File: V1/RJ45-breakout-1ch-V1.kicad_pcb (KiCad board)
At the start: 2 copper layers, 110 x 100 mm, 37 parts, among them J1 RJ45, J2 SWITCHES

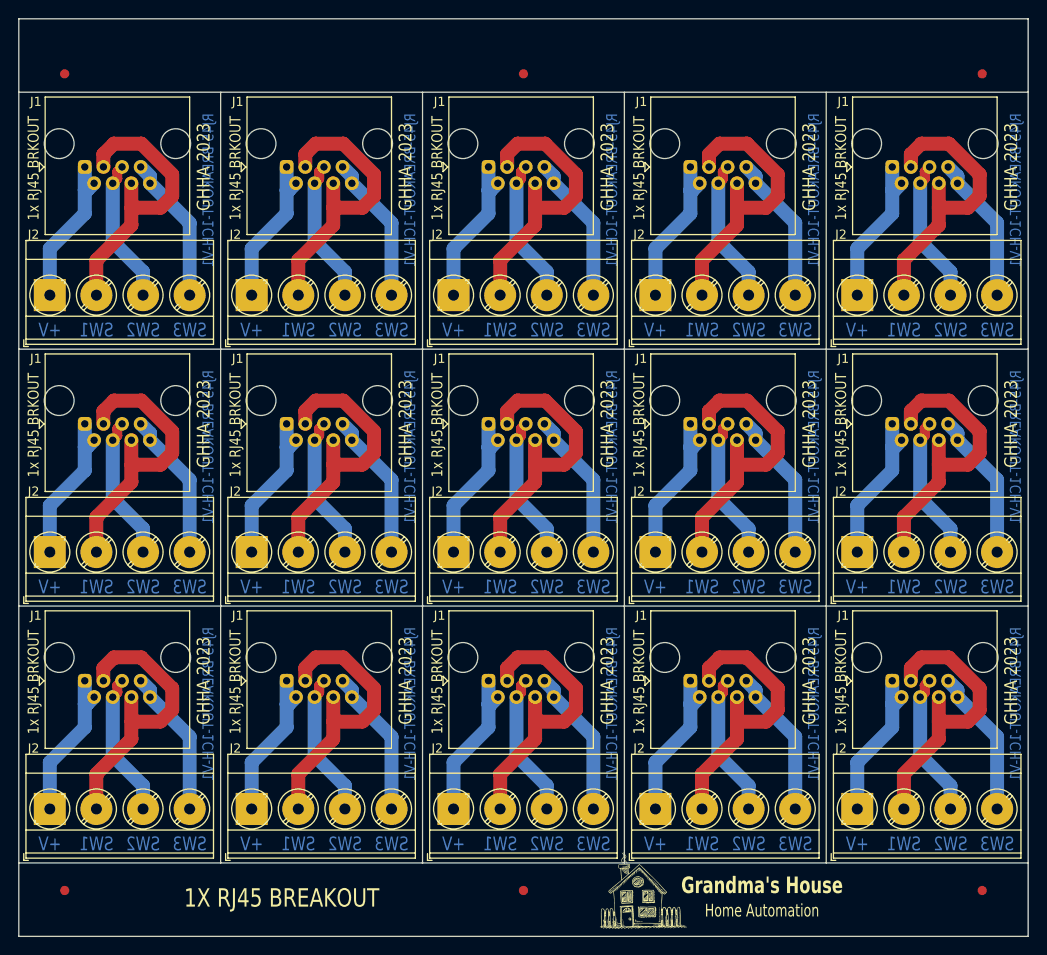
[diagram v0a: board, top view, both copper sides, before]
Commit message: Footprints updated
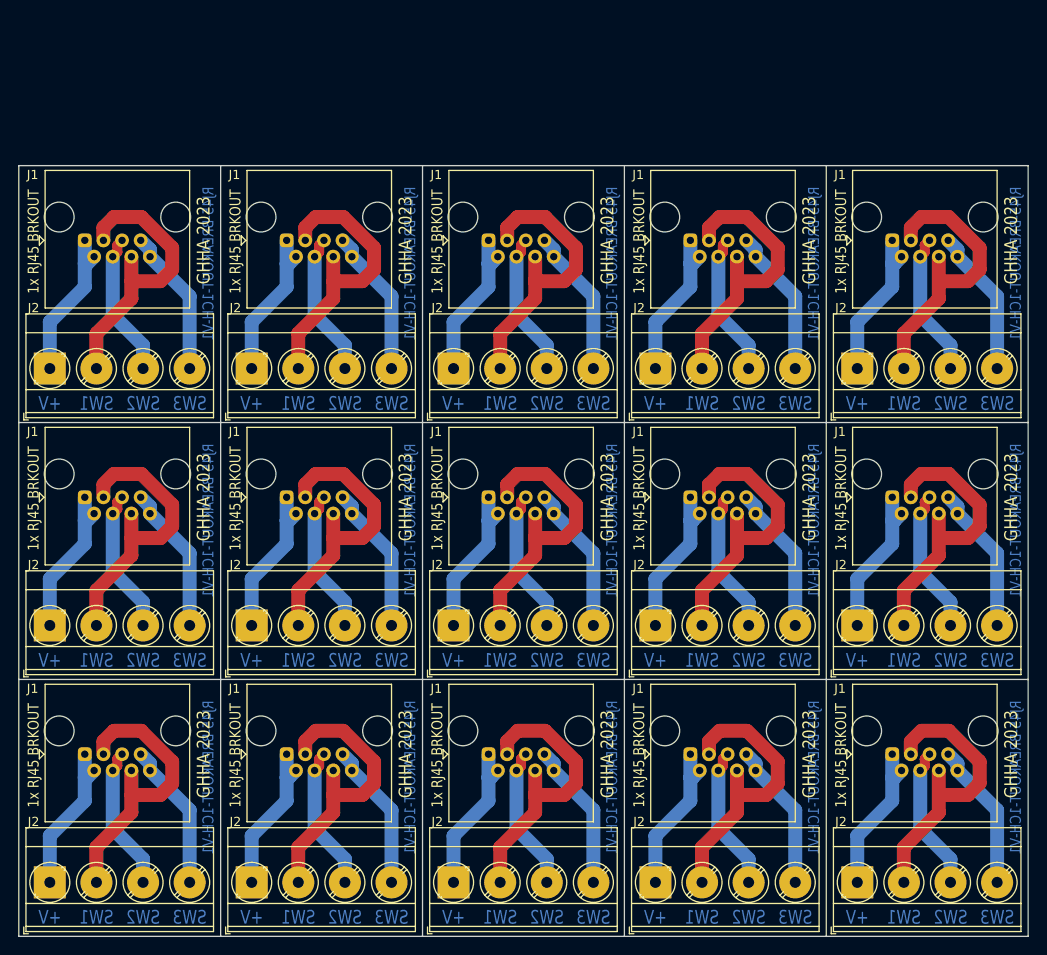
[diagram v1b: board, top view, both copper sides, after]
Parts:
- removed ?: , Tales:Grandmas_small
- removed FID1, FID2, FID3, FID4, FID5, FID6: Fiducial_1mm_Mask2mm, Fiducial:Fiducial_1mm_Mask2mm
- J1 (x15): footprint Tales:RJ45_Amphenol_RJHSE5080 -> Tales:RJ45_CKMTW_R-RJ45R08P-A004
- moved J2 8.00 mm to (186.4, 134.1)
- moved J2 8.00 mm to (98.4, 134.1)
- moved J2 8.00 mm to (164.4, 134.1)
- moved J2 8.00 mm to (142.4, 134.1)
- moved J2 8.00 mm to (120.4, 134.1)
- moved J1 8.00 mm to (102.2, 120.1)
- moved J1 8.00 mm to (146.2, 92.1)
- moved J1 8.00 mm to (124.2, 120.1)
- moved J1 8.00 mm to (124.2, 92.1)
- moved J1 8.00 mm to (190.2, 120.1)
- moved J1 8.00 mm to (190.2, 92.1)
- moved J1 8.00 mm to (102.2, 92.1)
- moved J1 8.00 mm to (168.2, 120.1)
- moved J1 8.00 mm to (168.2, 92.1)
- moved J1 8.00 mm to (146.2, 120.1)
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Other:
- board size 110 x 100 mm -> 110 x 84 mm
- board text added: "V-CUT"
- board text removed: "1X RJ45 BREAKOUT"
- board text removed: "Grandma's House"
- board text removed: "Home Automation"
